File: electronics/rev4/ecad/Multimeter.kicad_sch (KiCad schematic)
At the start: 14 parts, among them J1 B1HSW6, SW1 SW_Push, U1 SC0915, U6 74HC164

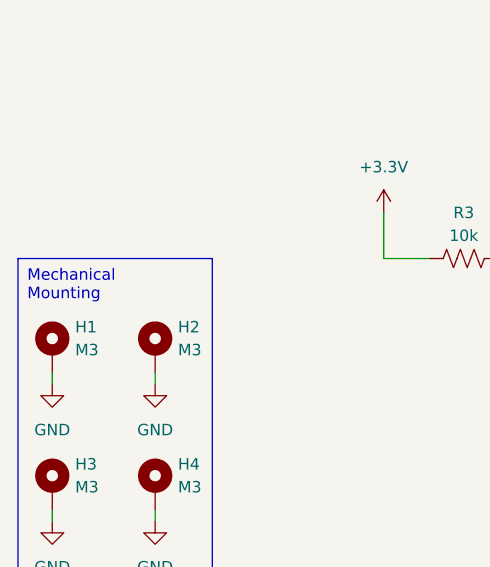
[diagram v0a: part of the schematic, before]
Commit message: started rev4
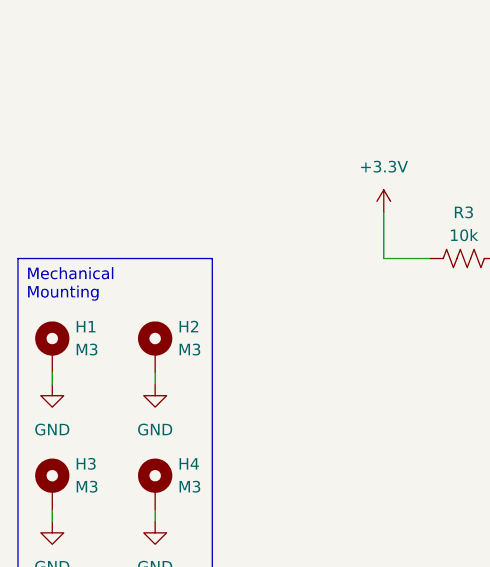
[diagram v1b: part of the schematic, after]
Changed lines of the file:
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@@
 (kicad_sch
-	(version 20231120)
+	(version 20250114)
 	(generator "eeschema")
-	(generator_version "8.0")
+	(generator_version "9.0")
 	(paper "USLetter")
 	(title_block
@@
 		(rev "2")
 	)
+	(text "Continuity/Diode Select"
+		(exclude_from_sim no)
+		(at 96.774 166.624 0)
+		(effects
+			(font
+				(size 1.27 1.27)
+			)
+		)
+	)
+	(text_box "Mechanical Mounting"
+		(exclude_from_sim no)
+		(at 16.51 161.29 0)
+		(size 21.59 36.83)
+		(margins 0.9525 0.9525 0.9525 0.9525)
+		(stroke
+			(width 0)
+			(type default)
+		)
+		(fill
+			(type none)
+		)
+		(effects
+			(font
+				(size 1.27 1.27)
+			)
+			(justify left top)
+		)
+	)
 	(junction
 		(at 151.13 48.26)
@@
 		)
 	)
-	(text_box "Mechanical Mounting"
-		(exclude_from_sim no)
-		(at 16.51 161.29 0)
-		(size 21.59 36.83)
-		(stroke
-			(width 0)
-			(type default)
-		)
-		(fill
-			(type none)
-		)
-		(effects
-			(font
-				(size 1.27 1.27)
-			)
-			(justify left top)
-		)
-	)
-	(text "Continuity/Diode Select"
-		(exclude_from_sim no)
-		(at 96.774 166.624 0)
-		(effects
-			(font
-				(size 1.27 1.27)
-			)
-		)
-	)
 	(symbol
 		(lib_id "power:+5V")
@@
 		)
 		(instances
-			(project ""
+			(project "Multimeter"
 				(path "/cb819000-1954-426e-958e-510a70bc03c7"
 					(reference "#PWR45")
@@
 		)
 		(instances
-			(project ""
+			(project "Multimeter"
 				(path "/cb819000-1954-426e-958e-510a70bc03c7"
 					(reference "#FLG1")
@@
 		)
 		(instances
-			(project ""
+			(project "Multimeter"
 				(path "/cb819000-1954-426e-958e-510a70bc03c7"
 					(reference "#PWR04")
@@
 		)
 		(instances
-			(project ""
+			(project "Multimeter"
 				(path "/cb819000-1954-426e-958e-510a70bc03c7"
 					(reference "D2")
@@
 		)
 		(instances
-			(project ""
+			(project "Multimeter"
 				(path "/cb819000-1954-426e-958e-510a70bc03c7"
 					(reference "C7")
@@
 		)
 		(instances
-			(project ""
+			(project "Multimeter"
 				(path "/cb819000-1954-426e-958e-510a70bc03c7"
 					(reference "R67")
@@
 		)
 		(instances
-			(project ""
+			(project "Multimeter"
 				(path "/cb819000-1954-426e-958e-510a70bc03c7"
 					(reference "D6")
@@
 		)
 		(instances
-			(project ""
+			(project "Multimeter"
 				(path "/cb819000-1954-426e-958e-510a70bc03c7"
 					(reference "U1")
@@
 		)
 		(instances
-			(project ""
+			(project "Multimeter"
 				(path "/cb819000-1954-426e-958e-510a70bc03c7"
 					(reference "#PWR3")
@@
 		)
 		(instances
-			(project ""
+			(project "Multimeter"
 				(path "/cb819000-1954-426e-958e-510a70bc03c7"
 					(reference "SW1")
@@
 		)
 		(instances
-			(project ""
+			(project "Multimeter"
 				(path "/cb819000-1954-426e-958e-510a70bc03c7"
 					(reference "U6")
@@
 		)
 		(instances
-			(project ""
+			(project "Multimeter"
 				(path "/cb819000-1954-426e-958e-510a70bc03c7"
 					(reference "#FLG3")
@@
 		)
 		(instances
-			(project ""
+			(project "Multimeter"
 				(path "/cb819000-1954-426e-958e-510a70bc03c7"
 					(reference "J1")
@@
 		)
 		(instances
-			(project ""
+			(project "Multimeter"
 				(path "/cb819000-1954-426e-958e-510a70bc03c7"
 					(reference "F1")
@@
 		)
 		(instances
-			(project ""
+			(project "Multimeter"
 				(path "/cb819000-1954-426e-958e-510a70bc03c7"
 					(reference "#PWR44")
@@
 		(at 36.83 66.04)
 		(size 25.4 48.26)
+		(exclude_from_sim no)
+		(in_bom yes)
+		(on_board yes)
+		(dnp no)
 		(fields_autoplaced yes)
 		(stroke
@@
 		(at 203.2 60.96)
 		(size 38.1 86.36)
+		(exclude_from_sim no)
+		(in_bom yes)
+		(on_board yes)
+		(dnp no)
 		(fields_autoplaced yes)
 		(stroke
@@
 		)
 	)
+	(embedded_fonts no)
 )
